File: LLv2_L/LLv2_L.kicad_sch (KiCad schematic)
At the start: 10 parts, among them IC1 TEENSY_4.0, J1 AudioJack4

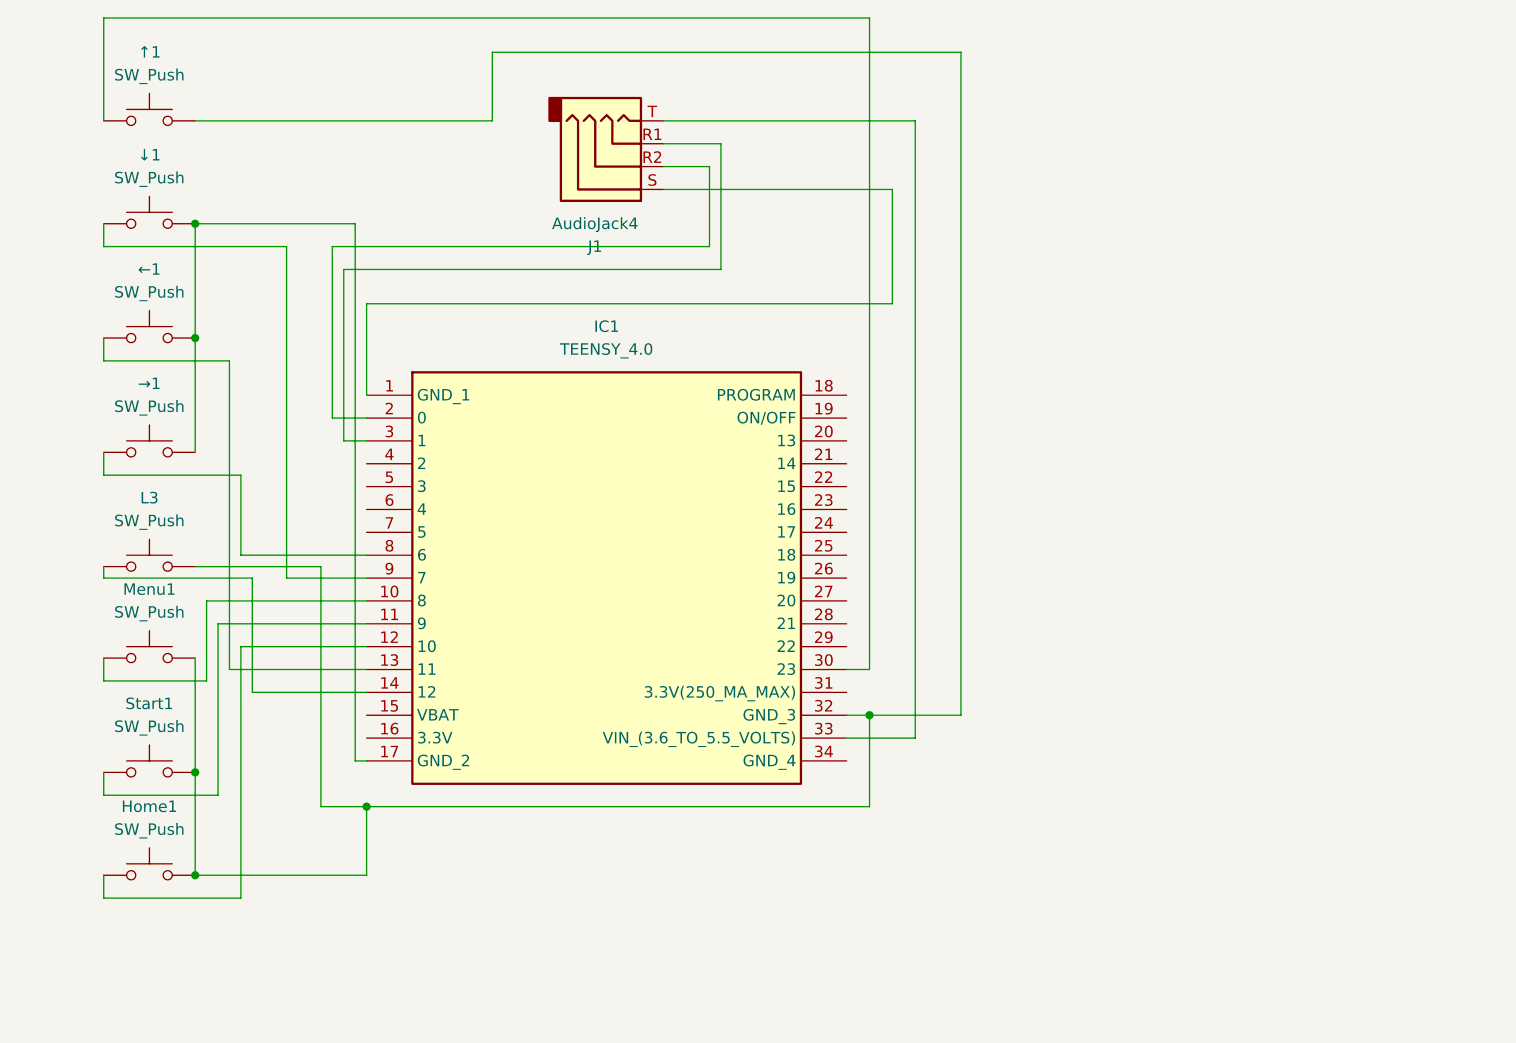
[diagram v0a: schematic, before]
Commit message: Update Softwere
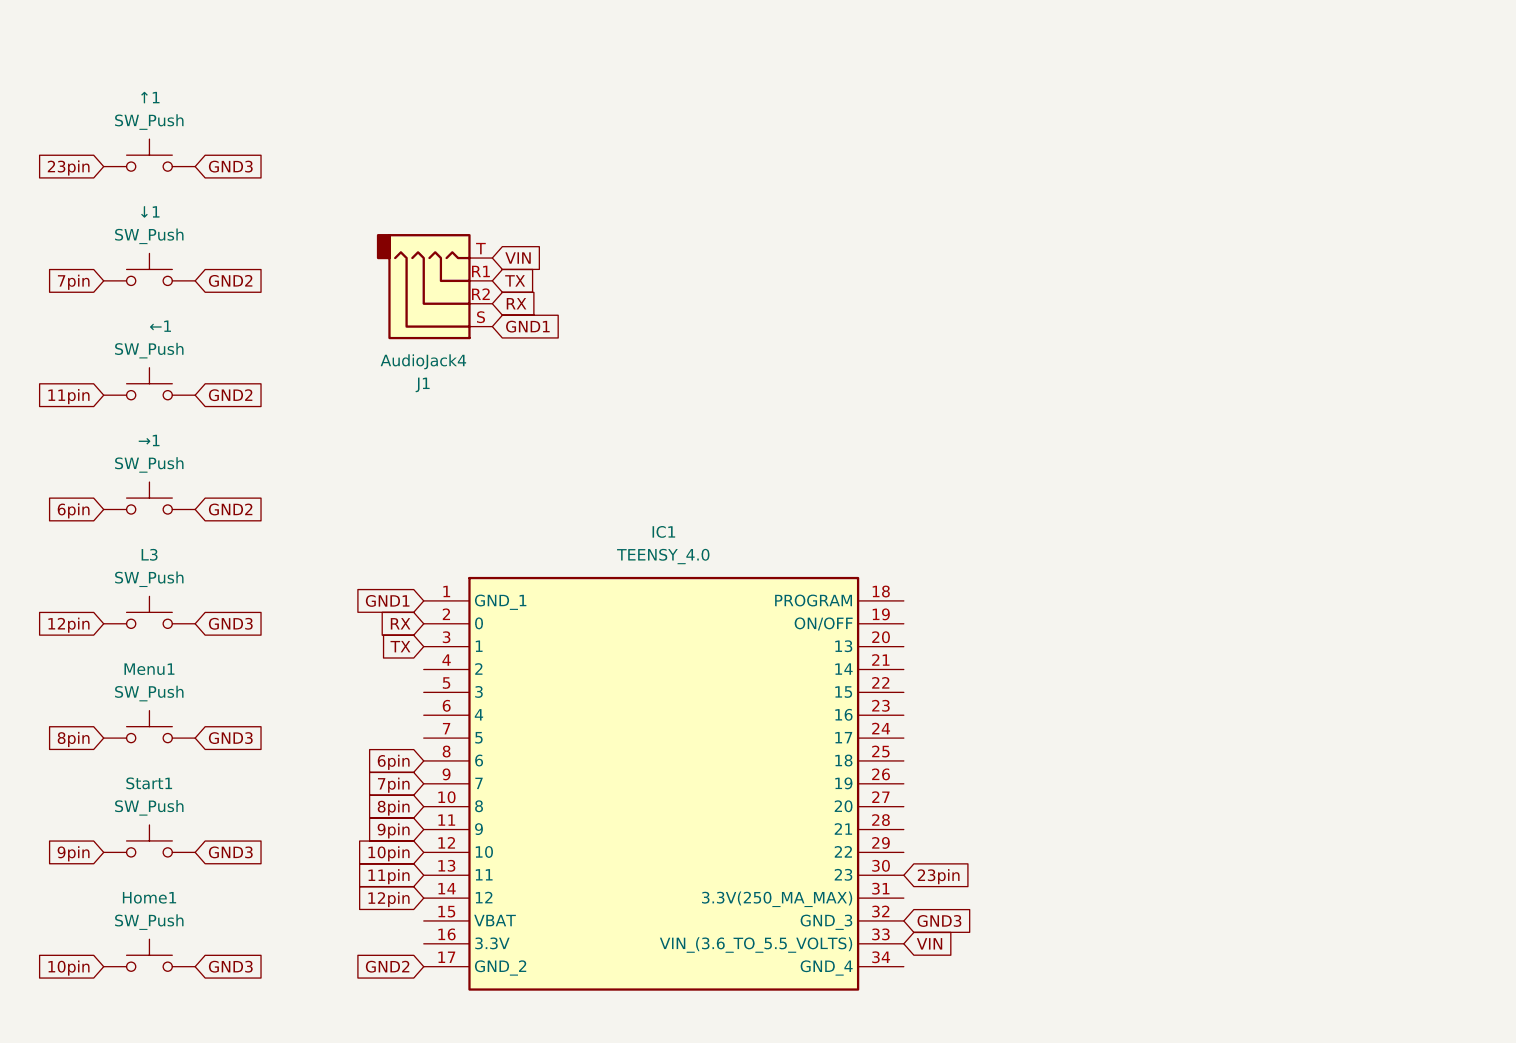
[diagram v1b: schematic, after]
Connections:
- net GND3: now reaches Home1.1, IC1.32 (GND_3), L3.2, Menu1.1, Start1.1, ↑1.2
- net 8pin: now reaches IC1.10 (8), Menu1.2
- net 9pin: now reaches IC1.11 (9), Start1.2
- net 7pin: now reaches IC1.9 (7), ↓1.1
- net GND2: now reaches IC1.17 (GND_2), ←1.2, →1.2, ↓1.2
- net 23pin: now reaches IC1.30 (23), ↑1.1
- net 10pin: now reaches Home1.2, IC1.12 (10)
- net 12pin: now reaches IC1.14 (12), L3.1
- net GND1: now reaches IC1.1 (GND_1), J1.S
- net 11pin: now reaches IC1.13 (11), ←1.1
- net RX: now reaches IC1.2 (0), J1.R2
- net TX: now reaches IC1.3 (1), J1.R1
- net VIN: now reaches IC1.33 (VIN_(3.6_TO_5.5_VOLTS)), J1.T
- net 6pin: now reaches IC1.8 (6), →1.1
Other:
- moved on the sheet: Home1, IC1, J1, L3, Menu1, Start1, ←1, ↑1, →1, ↓1

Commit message: add test script
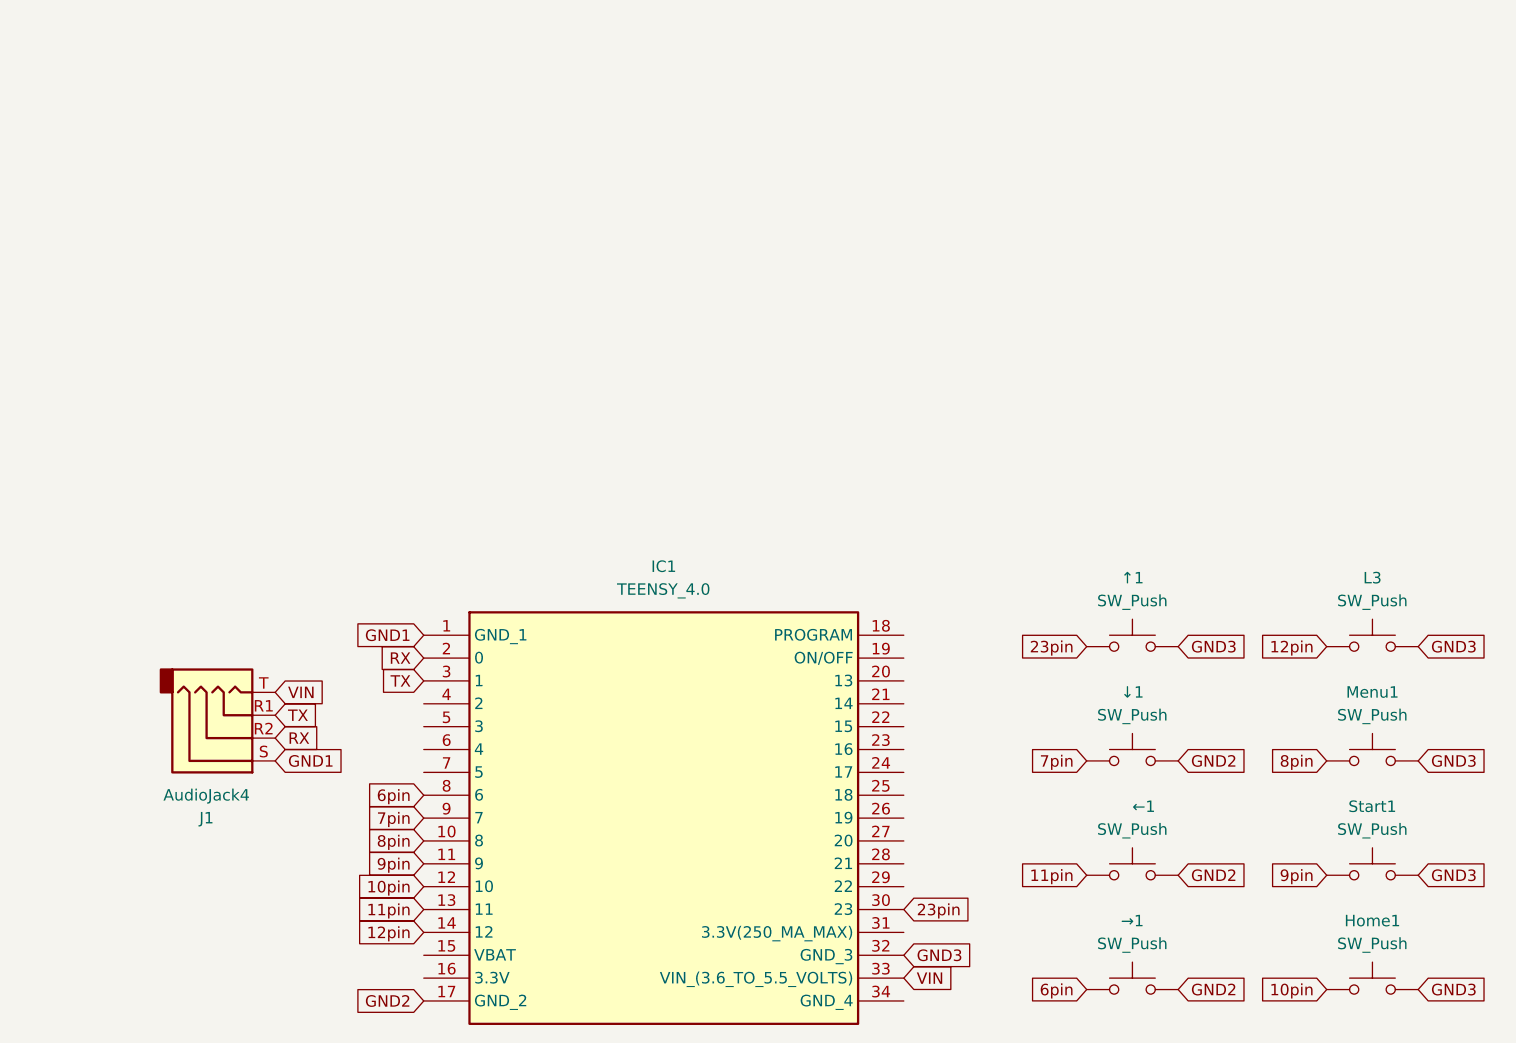
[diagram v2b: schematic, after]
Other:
- moved on the sheet: Home1, IC1, J1, L3, Menu1, Start1, ←1, ↑1, →1, ↓1
